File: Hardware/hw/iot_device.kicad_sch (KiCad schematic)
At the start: 36 parts, among them J2 USB4085-GF-A_REVA4, J4 Conn_01x04_Pin, Q1 PMOS, Q7 PMOS, SW1 SW_Push, SW2 SW_Push, U1 ESP32-C6-WROOM-1, U2 RV-3028-C7, U5 TPS63001, U9 USBLC6-4SC6

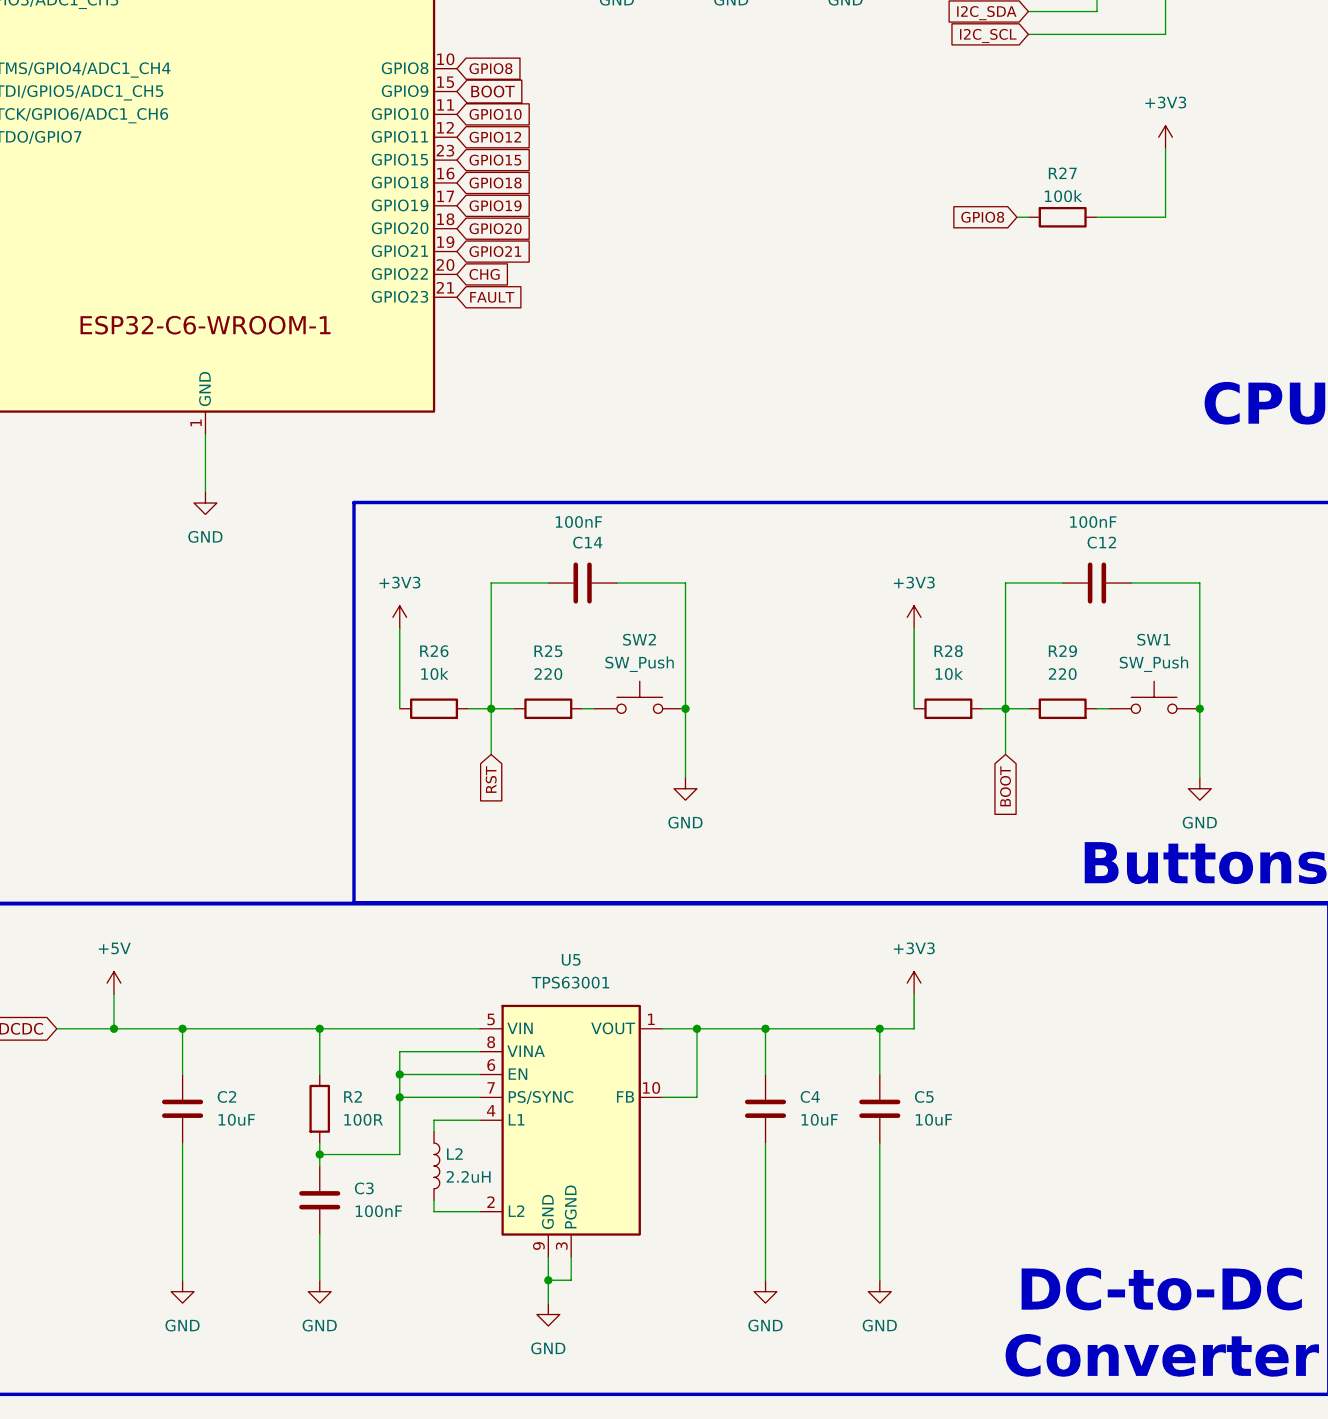
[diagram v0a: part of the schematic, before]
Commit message: little update
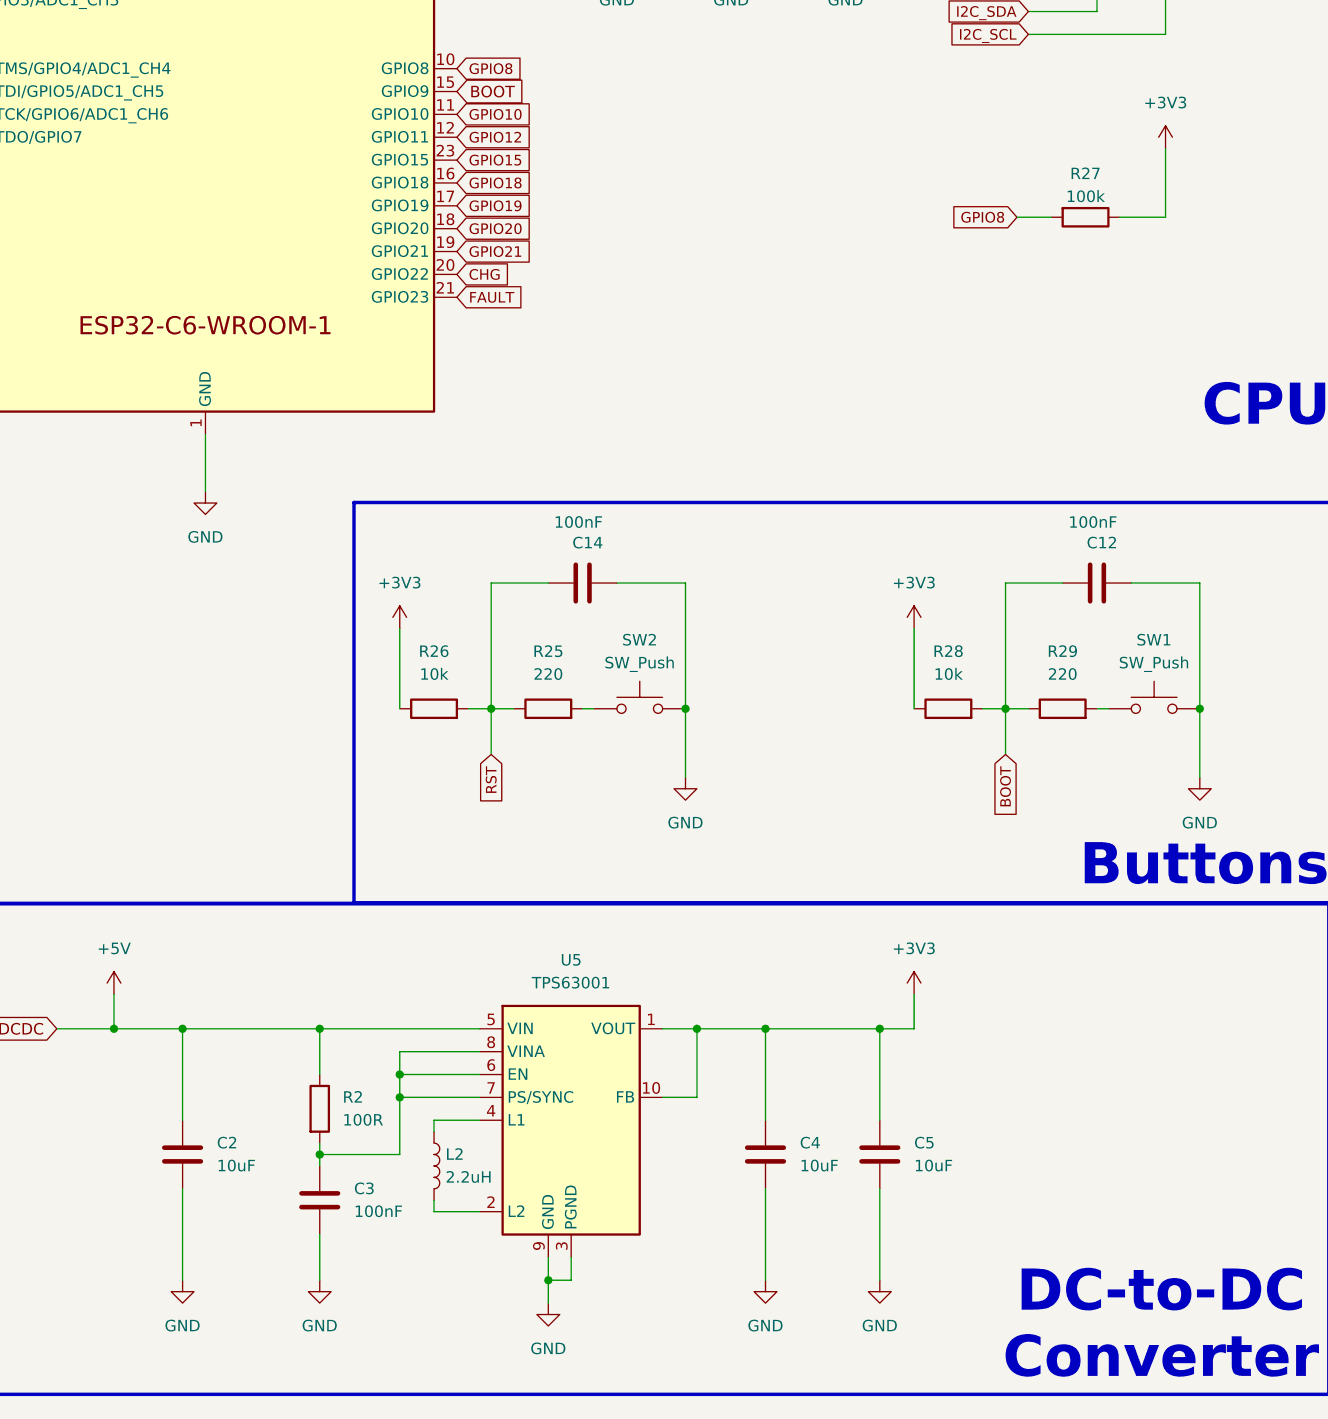
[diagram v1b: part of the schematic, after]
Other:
- moved on the sheet: C2, C4, C5, R27
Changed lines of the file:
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@@
 	(wire
 		(pts
-			(xy 49.53 157.48) (xy 49.53 162.56)
+			(xy 49.53 157.48) (xy 49.53 167.64)
 		)
 		(stroke
@@
 	(wire
 		(pts
-			(xy 142.24 67.31) (xy 143.51 67.31)
+			(xy 142.24 67.31) (xy 146.05 67.31)
 		)
 		(stroke
@@
 	(wire
 		(pts
-			(xy 114.3 157.48) (xy 114.3 162.56)
+			(xy 114.3 157.48) (xy 114.3 167.64)
 		)
 		(stroke
@@
 	(wire
 		(pts
-			(xy 127 170.18) (xy 127 185.42)
+			(xy 127 175.26) (xy 127 185.42)
 		)
 		(stroke
@@
 	(wire
 		(pts
-			(xy 151.13 67.31) (xy 158.75 67.31)
+			(xy 153.67 67.31) (xy 158.75 67.31)
 		)
 		(stroke
@@
 	(wire
 		(pts
-			(xy 127 157.48) (xy 127 162.56)
+			(xy 127 157.48) (xy 127 167.64)
 		)
 		(stroke
@@
 	(wire
 		(pts
-			(xy 49.53 170.18) (xy 49.53 185.42)
+			(xy 49.53 175.26) (xy 49.53 185.42)
 		)
 		(stroke
@@
 	(wire
 		(pts
-			(xy 114.3 170.18) (xy 114.3 185.42)
+			(xy 114.3 175.26) (xy 114.3 185.42)
 		)
 		(stroke
@@
 	(symbol
 		(lib_id "Device:C")
-		(at 114.3 166.37 0)
+		(at 114.3 171.45 0)
 		(unit 1)
 		(exclude_from_sim no)
@@
 		(fields_autoplaced yes)
 		(property "Reference" "C4"
-			(at 118.11 165.0999 0)
+			(at 118.11 170.1799 0)
 			(effects
 				(font
@@
 		)
 		(property "Value" "10uF"
-			(at 118.11 167.6399 0)
+			(at 118.11 172.7199 0)
 			(effects
 				(font
@@
 		)
 		(property "Footprint" "Capacitor_SMD:C_0805_2012Metric"
-			(at 115.2652 170.18 0)
+			(at 115.2652 175.26 0)
 			(effects
 				(font
@@
 		)
 		(property "Datasheet" "~"
-			(at 114.3 166.37 0)
+			(at 114.3 171.45 0)
 			(effects
 				(font
@@
 		)
 		(property "Description" "Unpolarized capacitor"
-			(at 114.3 166.37 0)
+			(at 114.3 171.45 0)
 			(effects
 				(font
@@
 	(symbol
 		(lib_id "Device:C")
-		(at 127 166.37 0)
+		(at 127 171.45 0)
 		(unit 1)
 		(exclude_from_sim no)
@@
 		(fields_autoplaced yes)
 		(property "Reference" "C5"
-			(at 130.81 165.0999 0)
+			(at 130.81 170.1799 0)
 			(effects
 				(font
@@
 		)
 		(property "Value" "10uF"
-			(at 130.81 167.6399 0)
+			(at 130.81 172.7199 0)
 			(effects
 				(font
@@
 		)
 		(property "Footprint" "Capacitor_SMD:C_0805_2012Metric"
-			(at 127.9652 170.18 0)
+			(at 127.9652 175.26 0)
 			(effects
 				(font
@@
 		)
 		(property "Datasheet" "~"
-			(at 127 166.37 0)
+			(at 127 171.45 0)
 			(effects
 				(font
@@
 		)
 		(property "Description" "Unpolarized capacitor"
-			(at 127 166.37 0)
+			(at 127 171.45 0)
 			(effects
 				(font
@@
 	(symbol
 		(lib_id "Device:R")
-		(at 147.32 67.31 270)
+		(at 149.86 67.31 270)
 		(unit 1)
 		(exclude_from_sim no)
@@
 		(dnp no)
 		(property "Reference" "R27"
-			(at 147.32 62.484 90)
+			(at 149.86 62.484 90)
 			(effects
 				(font
@@
 		)
 		(property "Value" "100k"
-			(at 147.32 65.024 90)
+			(at 149.86 65.024 90)
 			(effects
 				(font
@@
 		)
 		(property "Footprint" "Resistor_SMD:R_0805_2012Metric"
-			(at 147.32 65.532 90)
+			(at 149.86 65.532 90)
 			(effects
 				(font
@@
 		)
 		(property "Datasheet" "~"
-			(at 147.32 67.31 0)
+			(at 149.86 67.31 0)
 			(effects
 				(font
@@
 		)
 		(property "Description" "Resistor"
-			(at 147.32 67.31 0)
+			(at 149.86 67.31 0)
 			(effects
 				(font
@@
 	(symbol
 		(lib_id "Device:C")
-		(at 49.53 166.37 0)
+		(at 49.53 171.45 0)
 		(unit 1)
 		(exclude_from_sim no)
@@
 		(fields_autoplaced yes)
 		(property "Reference" "C2"
-			(at 53.34 165.0999 0)
+			(at 53.34 170.1799 0)
 			(effects
 				(font
@@
 		)
 		(property "Value" "10uF"
-			(at 53.34 167.6399 0)
+			(at 53.34 172.7199 0)
 			(effects
 				(font
@@
 		)
 		(property "Footprint" "Capacitor_SMD:C_0805_2012Metric"
-			(at 50.4952 170.18 0)
+			(at 50.4952 175.26 0)
 			(effects
 				(font
@@
 		)
 		(property "Datasheet" "~"
-			(at 49.53 166.37 0)
+			(at 49.53 171.45 0)
 			(effects
 				(font
@@
 		)
 		(property "Description" "Unpolarized capacitor"
-			(at 49.53 166.37 0)
+			(at 49.53 171.45 0)
 			(effects
 				(font
